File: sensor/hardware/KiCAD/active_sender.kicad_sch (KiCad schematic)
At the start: 25 parts, among them J1 220V0, J2 Buzzer, J3 Water Sensor, Q1 AO3400A, SW1 SW_Push, SW2 SW_SPDT, U1 ESP32-C3_SUPERMINI_TH, U2 Ai-Thinker-Ra-02, U3 HLK-PM12

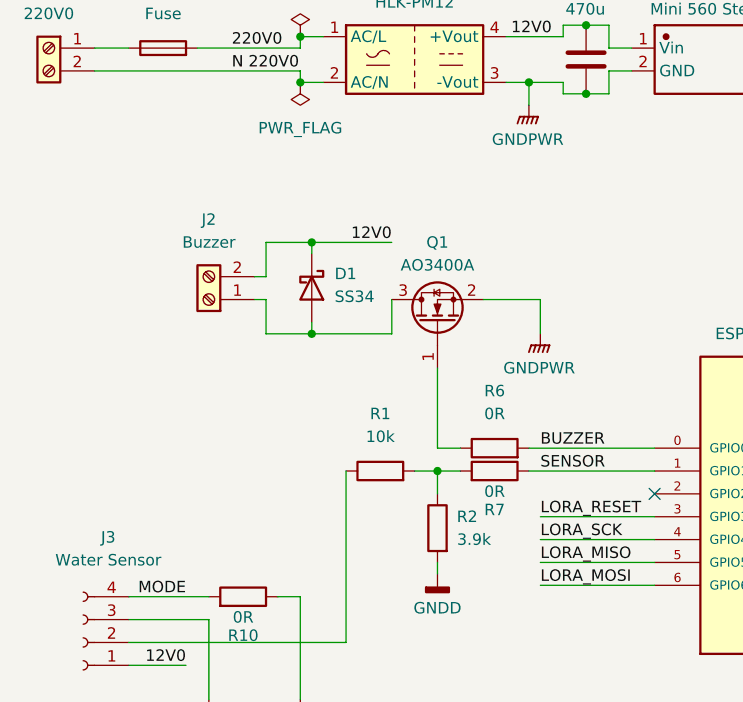
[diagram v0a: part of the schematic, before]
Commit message: sensor iteration 3
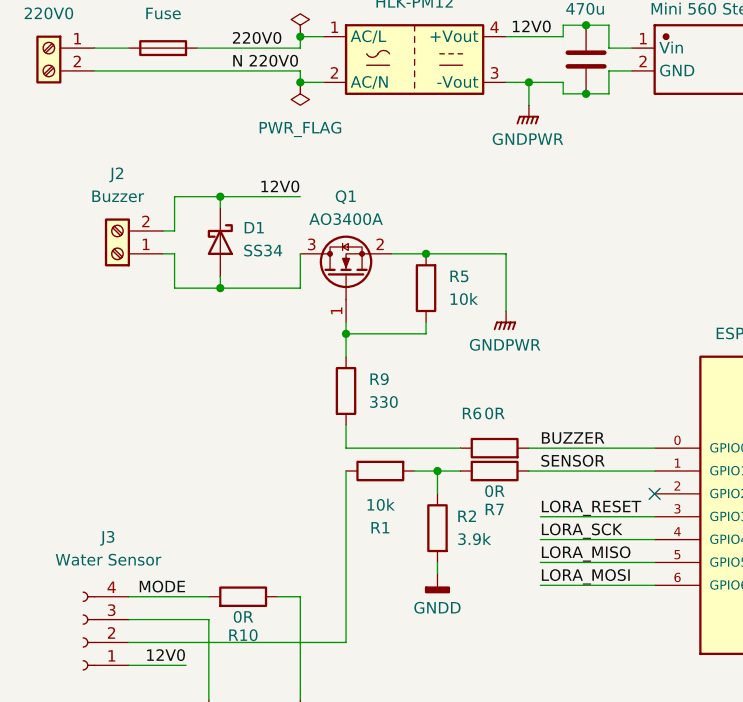
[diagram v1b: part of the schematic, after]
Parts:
- added R5: 10k, Resistor_SMD:R_1206_3216Metric_Pad1.30x1.75mm_HandSolder, symbol Device:R
- added R9: 330, Resistor_SMD:R_1206_3216Metric_Pad1.30x1.75mm_HandSolder, symbol Device:R
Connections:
- net GNDPWR: now also R5.2
- net at R6.1: now also R9.2; no longer Q1.1 (G)
- new net: Q1.1 (G), R5.1, R9.1
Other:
- moved on the sheet: D1, J2, Q1
